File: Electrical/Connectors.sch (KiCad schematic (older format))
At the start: 7 parts

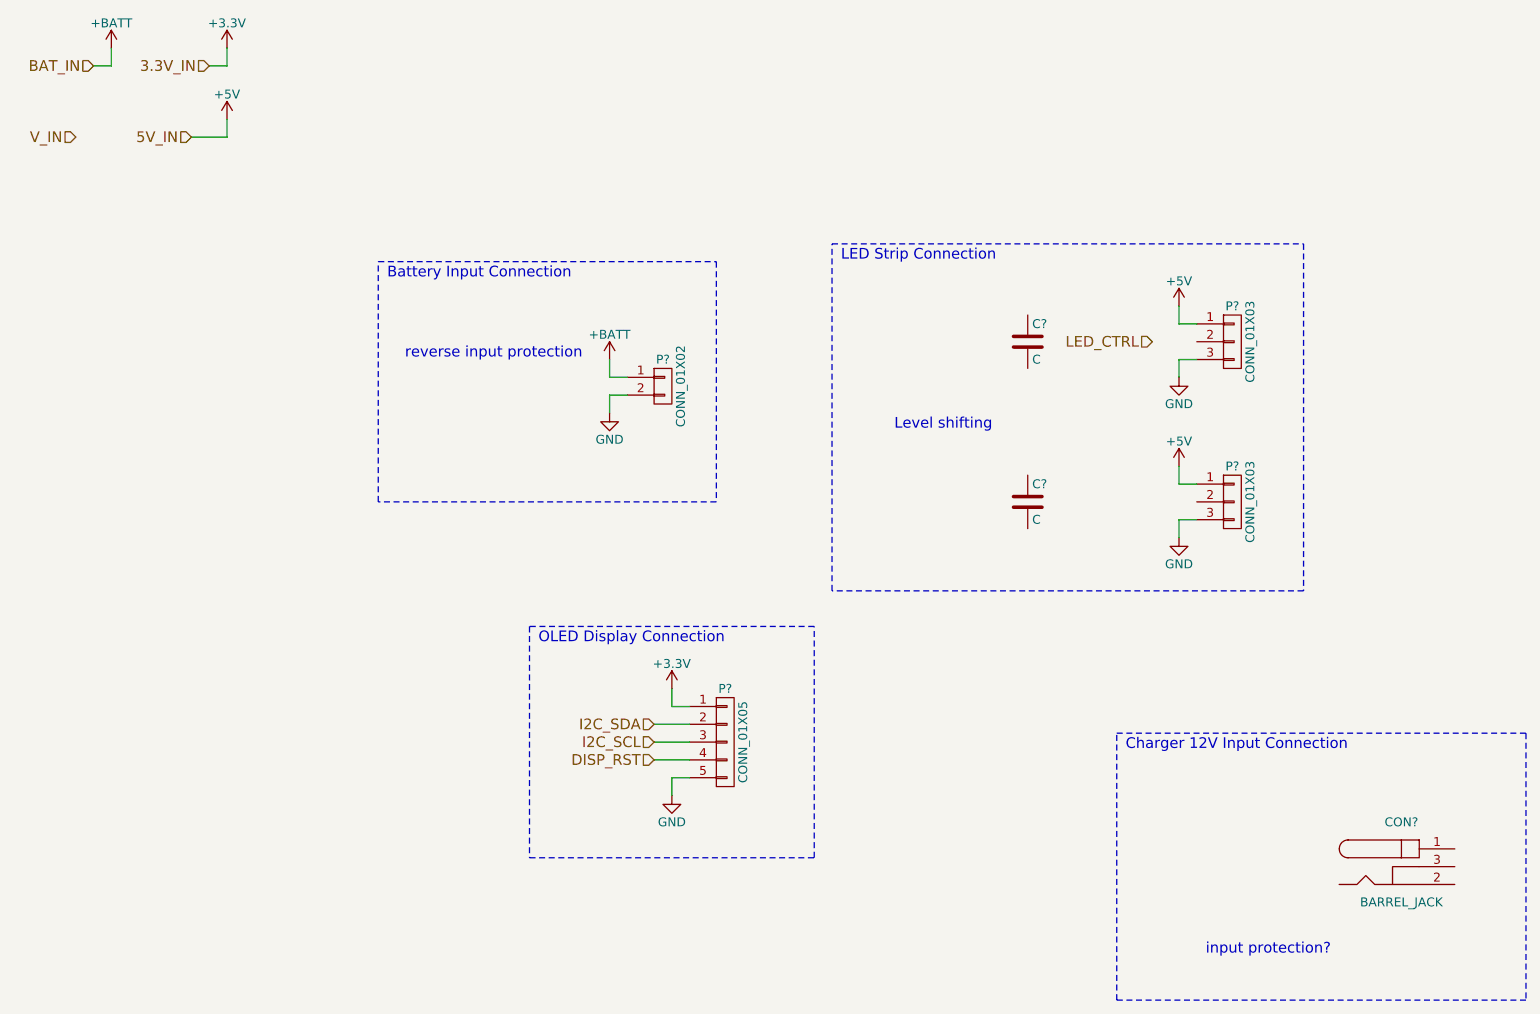
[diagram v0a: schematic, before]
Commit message: Continued work on schematic
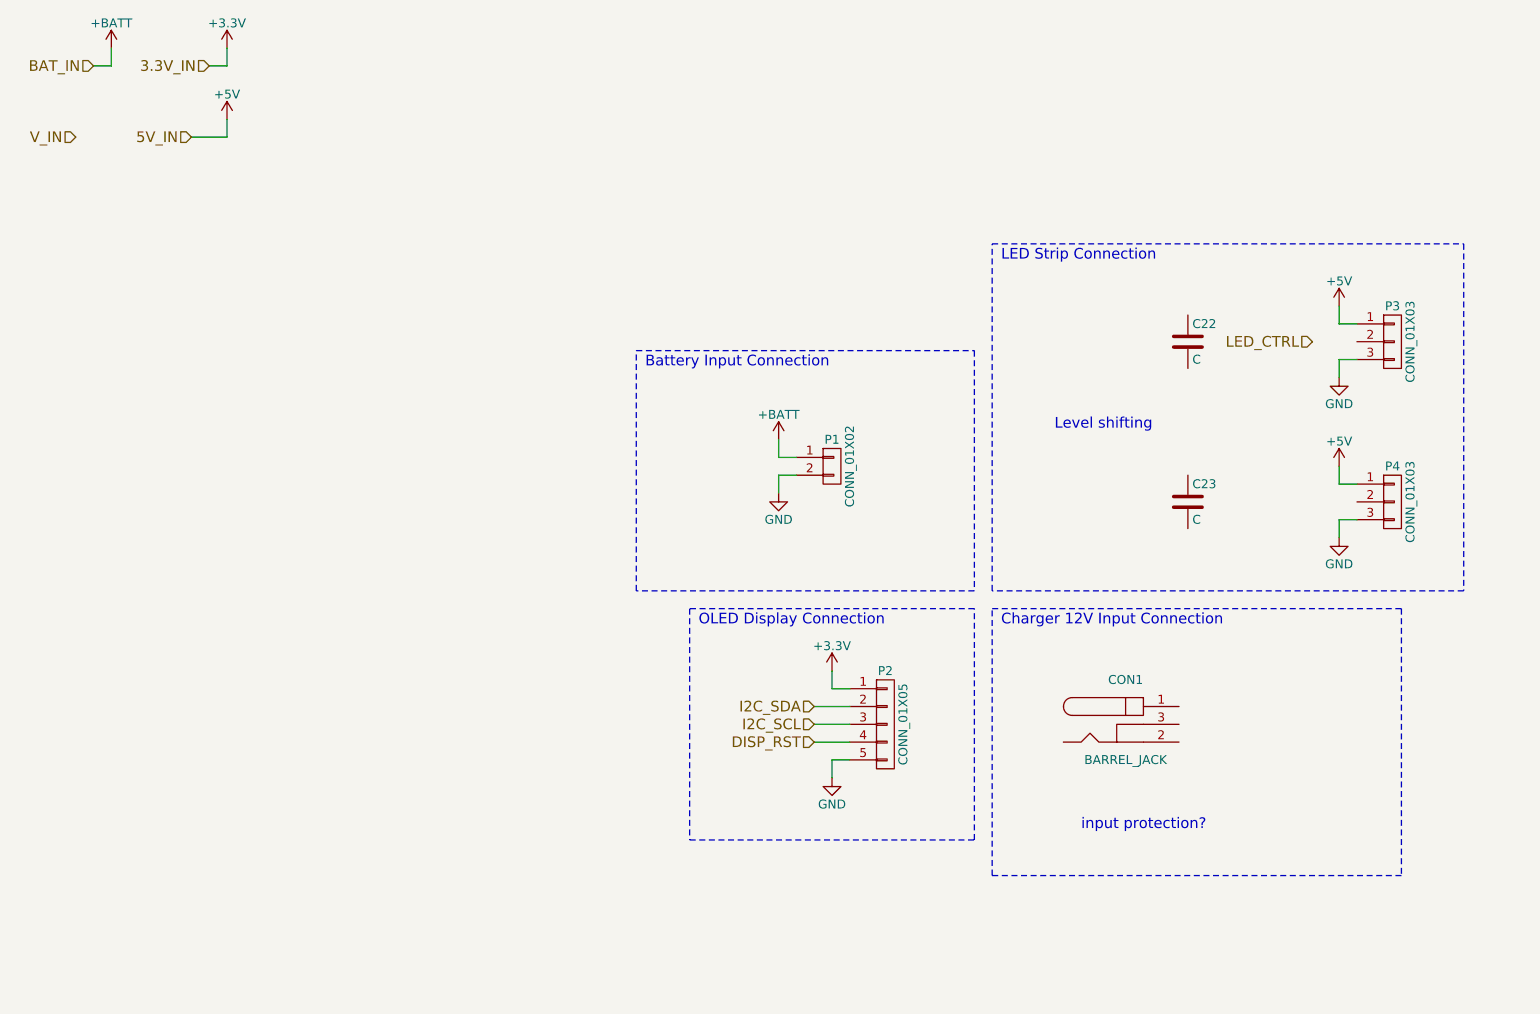
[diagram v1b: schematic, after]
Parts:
- gave numbers to parts that had none: 7
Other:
- note removed: "reverse input protection"
- moved on the sheet: C22, C23, CON1, P1, P2, P3, P4
